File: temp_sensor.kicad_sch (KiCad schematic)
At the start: 2 parts, among them U301 LMT87DCK

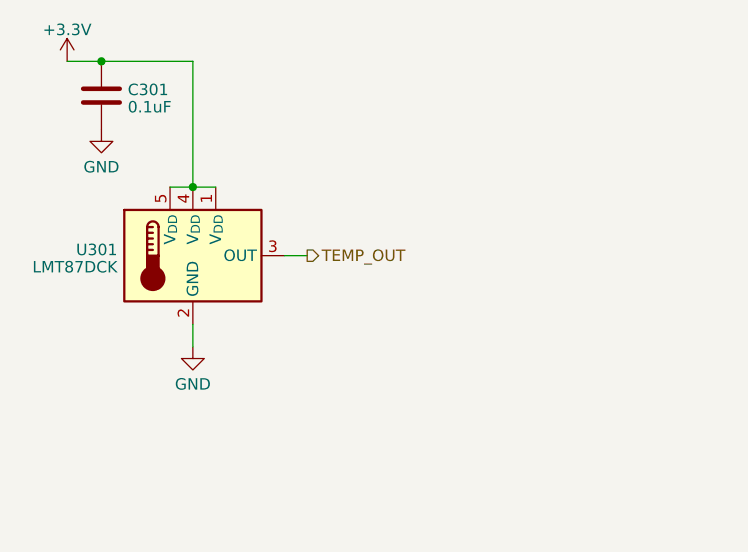
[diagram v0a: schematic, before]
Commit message: solar panel init
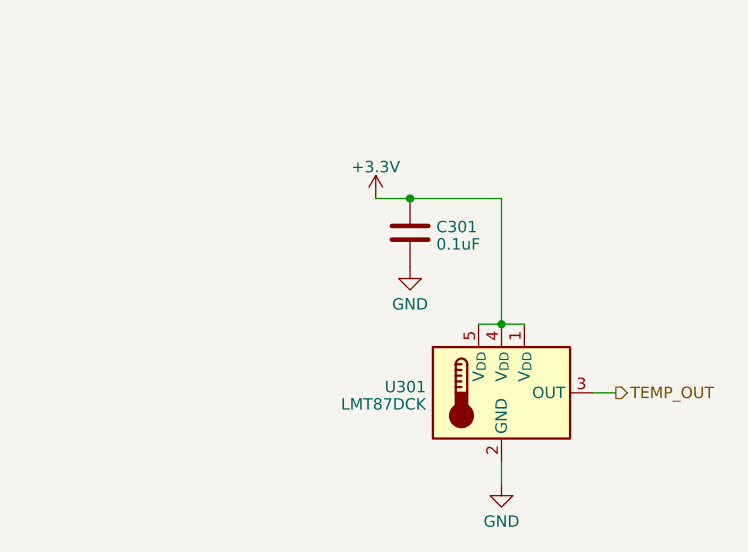
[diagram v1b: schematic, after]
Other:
- moved on the sheet: C301, U301
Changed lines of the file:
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@@
 (kicad_sch (version 20230121) (generator eeschema)
   (paper "A4")
-  (junction (at 115.57 74.93) (diameter 0) (color 0 0 0 0)
+  (junction (at 149.86 90.17) (diameter 0) (color 0 0 0 0)
   )
-  (junction (at 105.41 60.96) (diameter 0) (color 0 0 0 0)
+  (junction (at 139.7 76.2) (diameter 0) (color 0 0 0 0)
   )
-  (wire (pts (xy 105.41 60.96) (xy 115.57 60.96))
+  (wire (pts (xy 139.7 76.2) (xy 149.86 76.2))
     (stroke (width 0) (type default))
   )
-  (wire (pts (xy 101.6 60.96) (xy 105.41 60.96))
+  (wire (pts (xy 135.89 76.2) (xy 139.7 76.2))
     (stroke (width 0) (type default))
   )
-  (wire (pts (xy 115.57 90.17) (xy 115.57 92.71))
+  (wire (pts (xy 149.86 105.41) (xy 149.86 107.95))
     (stroke (width 0) (type default))
   )
-  (wire (pts (xy 125.73 82.55) (xy 128.27 82.55))
+  (wire (pts (xy 160.02 97.79) (xy 162.56 97.79))
     (stroke (width 0) (type default))
   )
-  (wire (pts (xy 115.57 74.93) (xy 115.57 60.96))
+  (wire (pts (xy 149.86 90.17) (xy 149.86 76.2))
     (stroke (width 0) (type default))
   )
-  (wire (pts (xy 115.57 74.93) (xy 118.11 74.93))
+  (wire (pts (xy 149.86 90.17) (xy 152.4 90.17))
     (stroke (width 0) (type default))
   )
-  (wire (pts (xy 113.03 74.93) (xy 115.57 74.93))
+  (wire (pts (xy 147.32 90.17) (xy 149.86 90.17))
     (stroke (width 0) (type default))
   )
-  (hierarchical_label "TEMP_OUT" (shape output) (at 128.27 82.55 0) (fields_autoplaced)
+  (hierarchical_label "TEMP_OUT" (shape output) (at 162.56 97.79 0) (fields_autoplaced)
     (effects (font (size 1.27 1.27)) (justify left))
   )
-  (symbol (lib_id "power:GND") (at 105.41 68.58 0) (unit 1)
+  (symbol (lib_id "power:GND") (at 139.7 83.82 0) (unit 1)
     (in_bom yes) (on_board yes) (dnp no) (fields_autoplaced)
-    (property "Reference" "#PWR0302" (at 105.41 74.93 0)
+    (property "Reference" "#PWR0302" (at 139.7 90.17 0)
       (effects (font (size 1.27 1.27)) hide)
     )
-    (property "Value" "GND" (at 105.41 72.7155 0)
+    (property "Value" "GND" (at 139.7 87.9555 0)
       (effects (font (size 1.27 1.27)))
     )
-    (property "Footprint" "" (at 105.41 68.58 0)
+    (property "Footprint" "" (at 139.7 83.82 0)
       (effects (font (size 1.27 1.27)) hide)
     )
-    (property "Datasheet" "" (at 105.41 68.58 0)
+    (property "Datasheet" "" (at 139.7 83.82 0)
       (effects (font (size 1.27 1.27)) hide)
     )
@@
     )
   )
-  (symbol (lib_id "Device:C") (at 105.41 64.77 0) (unit 1)
+  (symbol (lib_id "Device:C") (at 139.7 80.01 0) (unit 1)
     (in_bom yes) (on_board yes) (dnp no) (fields_autoplaced)
-    (property "Reference" "C301" (at 108.331 64.1263 0)
+    (property "Reference" "C301" (at 142.621 79.3663 0)
       (effects (font (size 1.27 1.27)) (justify left))
     )
-    (property "Value" "0.1uF" (at 108.331 66.0473 0)
+    (property "Value" "0.1uF" (at 142.621 81.2873 0)
       (effects (font (size 1.27 1.27)) (justify left))
     )
-    (property "Footprint" "Capacitor_SMD:C_0603_1608Metric_Pad1.08x0.95mm_HandSolder" (at 106.3752 68.58 0)
+    (property "Footprint" "Capacitor_SMD:C_0603_1608Metric_Pad1.08x0.95mm_HandSolder" (at 140.6652 83.82 0)
       (effects (font (size 1.27 1.27)) hide)
     )
-    (property "Datasheet" "~" (at 105.41 64.77 0)
+    (property "Datasheet" "~" (at 139.7 80.01 0)
       (effects (font (size 1.27 1.27)) hide)
     )
@@
     )
   )
-  (symbol (lib_id "Sensor_Temperature:LMT87DCK") (at 115.57 82.55 0) (unit 1)
+  (symbol (lib_id "Sensor_Temperature:LMT87DCK") (at 149.86 97.79 0) (unit 1)
     (in_bom yes) (on_board yes) (dnp no) (fields_autoplaced)
-    (property "Reference" "U301" (at 107.1881 81.9063 0)
+    (property "Reference" "U301" (at 141.4781 97.1463 0)
       (effects (font (size 1.27 1.27)) (justify right))
     )
-    (property "Value" "LMT87DCK" (at 107.1881 83.8273 0)
+    (property "Value" "LMT87DCK" (at 141.4781 99.0673 0)
       (effects (font (size 1.27 1.27)) (justify right))
     )
-    (property "Footprint" "Package_TO_SOT_SMD:SOT-353_SC-70-5" (at 115.57 92.71 0)
+    (property "Footprint" "Package_TO_SOT_SMD:SOT-353_SC-70-5" (at 149.86 107.95 0)
       (effects (font (size 1.27 1.27)) hide)
     )
-    (property "Datasheet" "http://www.ti.com/lit/ds/symlink/lmt87-q1.pdf" (at 115.57 82.55 0)
+    (property "Datasheet" "http://www.ti.com/lit/ds/symlink/lmt87-q1.pdf" (at 149.86 97.79 0)
       (effects (font (size 1.27 1.27)) hide)
     )
@@
     )
   )
-  (symbol (lib_id "power:GND") (at 115.57 92.71 0) (unit 1)
+  (symbol (lib_id "power:GND") (at 149.86 107.95 0) (unit 1)
     (in_bom yes) (on_board yes) (dnp no) (fields_autoplaced)
-    (property "Reference" "#PWR0303" (at 115.57 99.06 0)
+    (property "Reference" "#PWR0303" (at 149.86 114.3 0)
       (effects (font (size 1.27 1.27)) hide)
     )
-    (property "Value" "GND" (at 115.57 96.8455 0)
+    (property "Value" "GND" (at 149.86 112.0855 0)
       (effects (font (size 1.27 1.27)))
     )
-    (property "Footprint" "" (at 115.57 92.71 0)
+    (property "Footprint" "" (at 149.86 107.95 0)
       (effects (font (size 1.27 1.27)) hide)
     )
-    (property "Datasheet" "" (at 115.57 92.71 0)
+    (property "Datasheet" "" (at 149.86 107.95 0)
       (effects (font (size 1.27 1.27)) hide)
     )
@@
     )
   )
-  (symbol (lib_id "power:+3.3V") (at 101.6 60.96 0) (unit 1)
+  (symbol (lib_id "power:+3.3V") (at 135.89 76.2 0) (unit 1)
     (in_bom yes) (on_board yes) (dnp no) (fields_autoplaced)
-    (property "Reference" "#PWR0201" (at 101.6 64.77 0)
+    (property "Reference" "#PWR0201" (at 135.89 80.01 0)
       (effects (font (size 1.27 1.27)) hide)
     )
-    (property "Value" "+3.3V" (at 101.6 57.4581 0)
+    (property "Value" "+3.3V" (at 135.89 72.6981 0)
       (effects (font (size 1.27 1.27)))
     )
-    (property "Footprint" "" (at 101.6 60.96 0)
+    (property "Footprint" "" (at 135.89 76.2 0)
       (effects (font (size 1.27 1.27)) hide)
     )
-    (property "Datasheet" "" (at 101.6 60.96 0)
+    (property "Datasheet" "" (at 135.89 76.2 0)
       (effects (font (size 1.27 1.27)) hide)
     )
